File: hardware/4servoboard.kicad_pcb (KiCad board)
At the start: 2 copper layers, 22.9 x 23.6 mm, 34 parts, among them J1 USB_C_Receptacle, J2 PWM, J3 UART, J4 GND, J5 V_SERVO, J6 POWER, J7 DEBUG, U1 CH32X035F7P6, U2 XC6206P332MR

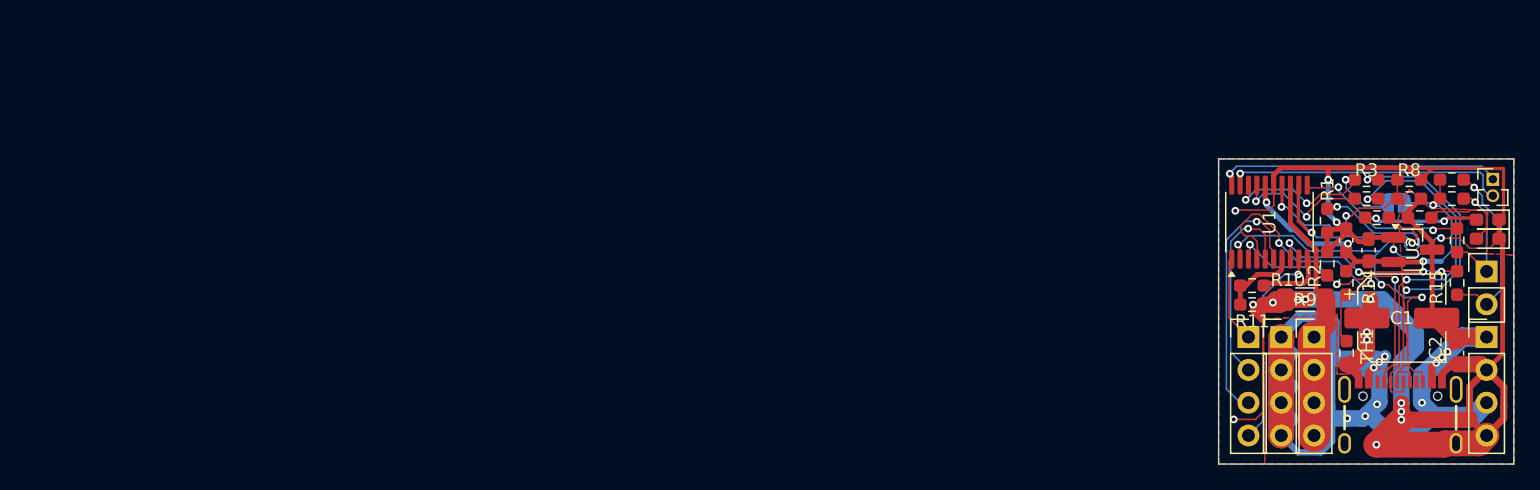
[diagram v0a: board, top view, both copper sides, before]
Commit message: wip: Rev0.4への更新
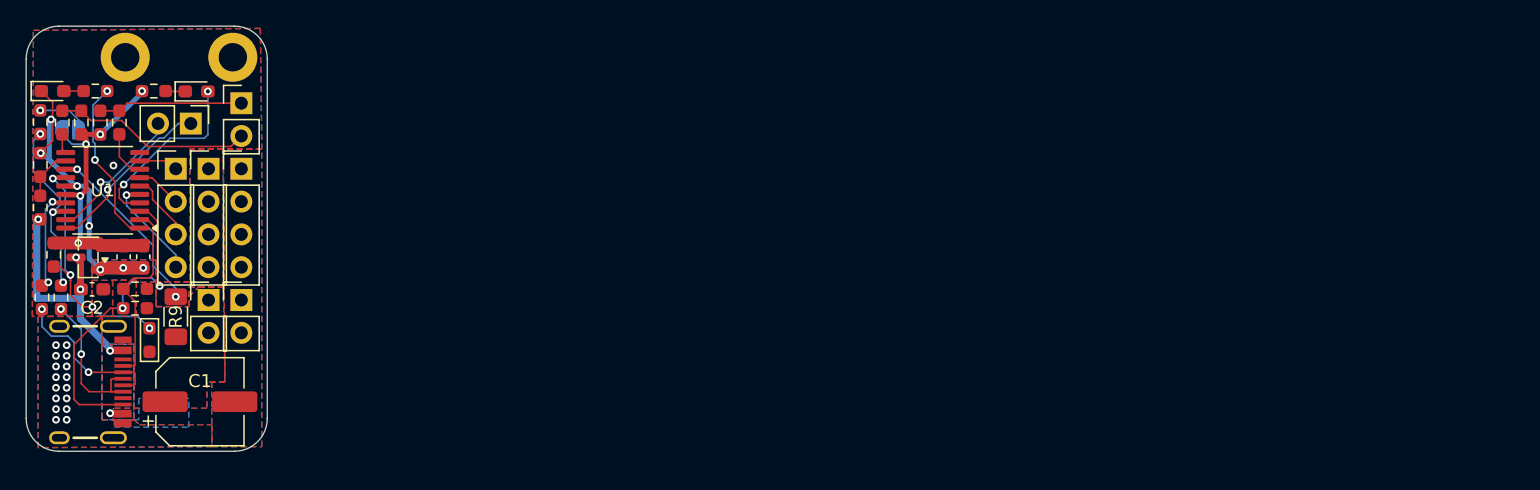
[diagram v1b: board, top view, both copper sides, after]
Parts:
- removed D1: SERVO_PWR, LED_SMD:LED_0603_1608Metric_Pad1.05x0.95mm_HandSolder
- removed QR*****: qr-uart-fscb, qr:qr-uart-fscb
- removed R11: 5.1k, Resistor_SMD:R_0603_1608Metric_Pad0.98x0.95mm_HandSolder
- removed R5: 1k, Resistor_SMD:R_0603_1608Metric_Pad0.98x0.95mm_HandSolder
- added D3: MCU_LED2, LED_SMD:LED_0603_1608Metric_Pad1.05x0.95mm_HandSolder, F.Cu at (127.9, 57.0)
- added J8: DEBUG, Connector_PinHeader_2.54mm:PinHeader_1x02_P2.54mm_Vertical, F.Cu at (127.4, 59.5)
- added R17: 5k1, Resistor_SMD:R_0603_1608Metric_Pad0.98x0.95mm_HandSolder, F.Cu at (115.7, 59.4)
- added REF**: MountingHole_2.2mm_M2_DIN965_Pad, MountingHole:MountingHole_2.2mm_M2_DIN965_Pad, F.Cu at (122.3, 54.4)
- added REF**: MountingHole_2.2mm_M2_DIN965_Pad, MountingHole:MountingHole_2.2mm_M2_DIN965_Pad, F.Cu at (130.7, 54.4)
- D2: value MCU_LED -> MCU_LED1
- J1: footprint PCM_SparkFun-Connector:USB-C_16 -> Download_Lib:USB-C_16-HandSolder
- J6: value POWER -> VBUS; footprint Connector_PinHeader_2.54mm:PinHeader_1x04_P2.54mm_Vertical -> Connector_PinHeader_2.54mm:PinHeader_1x02_P2.54mm_Vertical
- J7: value DEBUG -> GND; footprint Connector_PinHeader_1.27mm:PinHeader_1x02_P1.27mm_Vertical -> Connector_PinHeader_2.54mm:PinHeader_1x02_P2.54mm_Vertical
- R10: value 120k -> 1k
- R12, R13: value 1k -> 5k1
- R14, R8: value 5.1k -> 5k1
- R15, R16: value 1k -> 22
- TH1: value Thermistor_NTC -> 22k/B4050/NTC; footprint Resistor_SMD:R_0603_1608Metric_Pad0.98x0.95mm_HandSolder -> PCM_Resistor_SMD_AKL:R_0603_1608Metric_Pad0.98x0.95mm_HandSolder
- U2: footprint Package_TO_SOT_SMD:SOT-23_Handsoldering -> Package_TO_SOT_SMD:SOT-23
- moved D2 111.6 mm to (116.7, 57.0), turned to 0 degrees
- moved R15 108.7 mm to (117.4, 59.4), turned to -90 degrees
- moved R13 106.2 mm to (118.9, 59.4), turned to 90 degrees
- moved R8 106.0 mm to (115.7, 62.7), turned to 90 degrees
- moved R7 106.0 mm to (115.7, 66.0), turned to 90 degrees
- moved C2 105.8 mm to (119.8, 72.3), turned to 180 degrees
- moved R12 104.8 mm to (120.4, 59.4), turned to 90 degrees
- moved R16 104.0 mm to (121.9, 59.4), turned to -90 degrees
- moved R4 102.8 mm to (115.9, 73.0), turned to 90 degrees
- moved JP1 102.8 mm to (118.1, 60.0), turned to 180 degrees
- moved U2 102.6 mm to (119.5, 69.9), turned to 180 degrees
- moved R3 101.5 mm to (117.3, 73.0), turned to 90 degrees
- moved R14 100.1 mm to (116.8, 69.6)
- moved J7 99.9 mm to (128.8, 73.2)
- moved R6 99.7 mm to (120.0, 57.0)
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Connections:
- net PWM2 renamed PWM2/ADC2
- J2 pad 1: PWM0 -> PWM0/ADC0
- J2 pad 2: PWM1 -> PWM1/ADC1
- J2 pad 4: PWM3 -> PWM3/ADC3
- J6 pad 2: GND -> VBUS
- J7 pad 1: SWCLK -> GND
- J7 pad 2: SWDIO -> GND
- JP1 pad 1: DP -> Net-(JP1-A)
- R10 pad 1: OPA_O -> VDD
- R10 pad 2: OPA_N -> Net-(D3-K)
- R14 pad 2: PC3 -> TEMP_SENCE
- R15 pad 2: TX2 -> UART_B
- R16 pad 2: TX4 -> UART_A
- R6 pad 2: MCU_LED -> MCU_LED1
- R7 pad 2: PB1 -> V_SENCE
- R8 pad 1: PB1 -> V_SENCE
- TH1 pad 1: PC3 -> TEMP_SENCE
- U1 pad 1: PWM0 -> MCU_LED1
- U1 pad 10: OPA_O -> unconnected-(U1-PA4-Pad10)
- U1 pad 11: TX4 -> UART_B
- U1 pad 12: MCU_LED -> V_SENCE
- U1 pad 14: PB1 -> TEMP_SENCE
- U1 pad 4: PC3 -> MCU_LED2
- U1 pad 5: PWM1 -> PWM3/ADC3
- U1 pad 7: OPA_N -> PWM1/ADC1
- U1 pad 8: TX2 -> UART_A
- U1 pad 9: PWM3 -> PWM0/ADC0
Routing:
- net GND: track 154.2 -> 28.4 mm, vias 17 -> 24
- net VBUS: track 119.0 -> 22.5 mm, vias 10 -> 5
- net PC3: track 22.8 -> 0.00 mm, vias 2 -> 0
- net CC1: track 37.3 -> 15.1 mm, vias 3 -> 0
- net TEMP_SENCE: track 0.00 -> 19.7 mm, vias 0 -> 4
- net Net-(J1-D--PadA7): track 28.5 -> 12.6 mm
- net MCU_LED: track 15.9 -> 0.00 mm, vias 2 -> 0
- net PWM3: track 15.9 -> 0.00 mm, vias 1 -> 0
- net PWM1: track 15.7 -> 0.00 mm, vias 1 -> 0
- net Net-(J1-D+-PadA6): track 27.4 -> 11.8 mm
- net TX2: track 15.3 -> 0.00 mm, vias 4 -> 0
- net PWM2/ADC2: track 20.3 -> 5.26 mm, vias 1 -> 0
- net MCU_LED2: track 0.00 -> 14.4 mm, vias 0 -> 2
- net PB1: track 14.2 -> 0.00 mm, vias 2 -> 0
- net TX4: track 13.5 -> 0.00 mm, vias 2 -> 0
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- added copper zone on B.Cu, net OPA_P
- added copper zone on F.Cu, net OPA_P
- added copper zone on B.Cu, net VBUS
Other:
- board size 22.9 x 23.6 mm -> 18.7 x 32.9 mm
- board text removed: "DLM(4.7k)"
- board text removed: "GND"
- board text removed: "Made by EsEhEhElp"
- board text removed: "PWM"
- board text removed: "SWCLK"
- board text removed: "SWDIO"
- board text removed: "UART-FSCB V0.3"
- board text removed: "UART0"
- board text removed: "UART1"
- board text removed: "VBUS"
